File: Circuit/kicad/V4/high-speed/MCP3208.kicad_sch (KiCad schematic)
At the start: 15 parts, among them J16 Conn_01x02_Pin, J17 Conn_01x02_Pin, J18 Conn_01x02_Pin, J19 Conn_01x02_Pin, J20 Conn_01x02_Pin, J21 Conn_01x02_Pin, U24 MCP3208

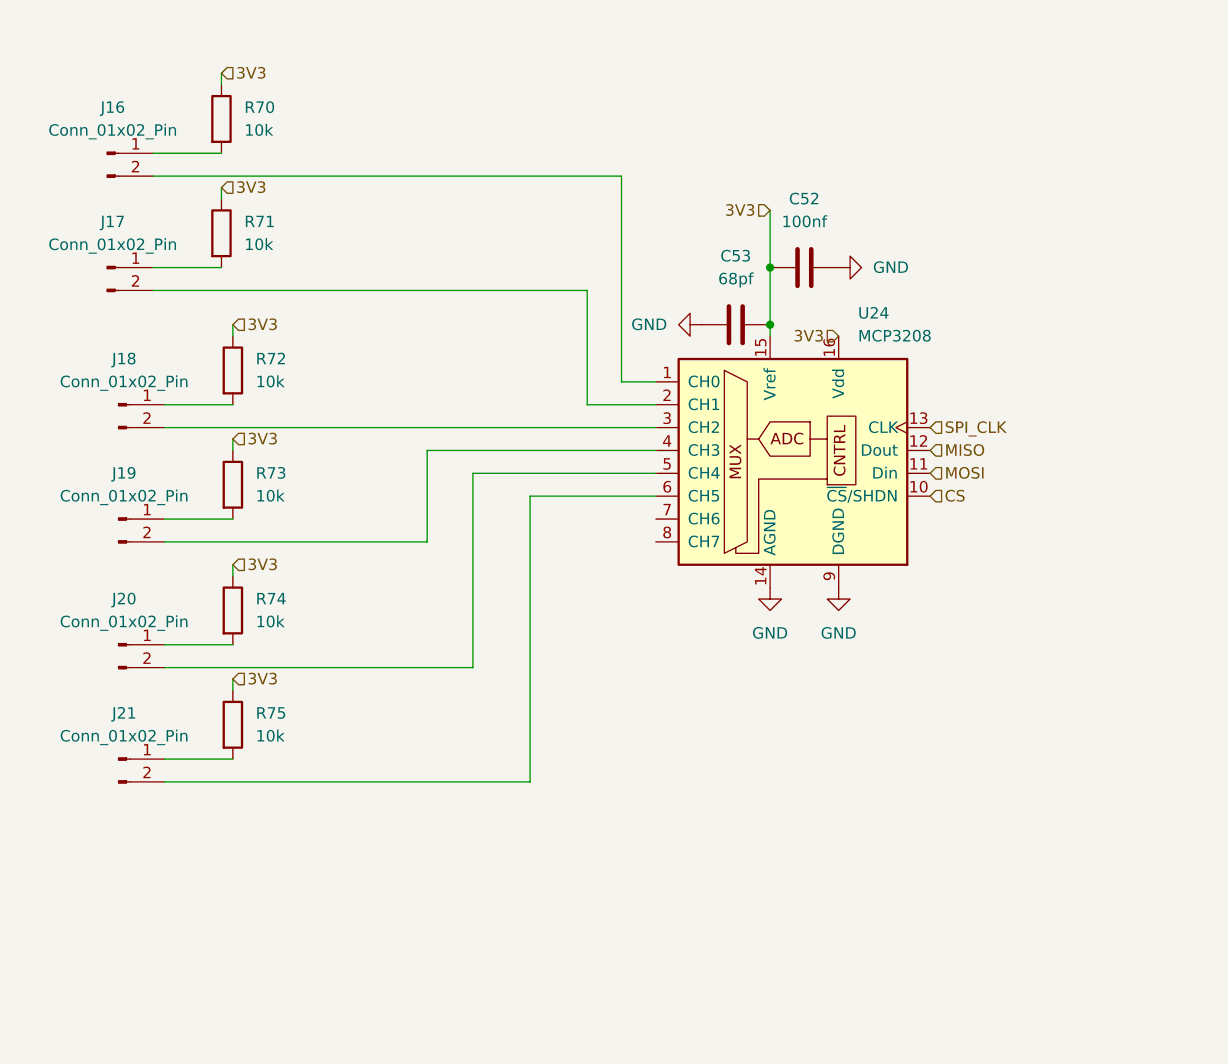
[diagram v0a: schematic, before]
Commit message: kicad: high speed V2.2 Circuit finish psu bom update
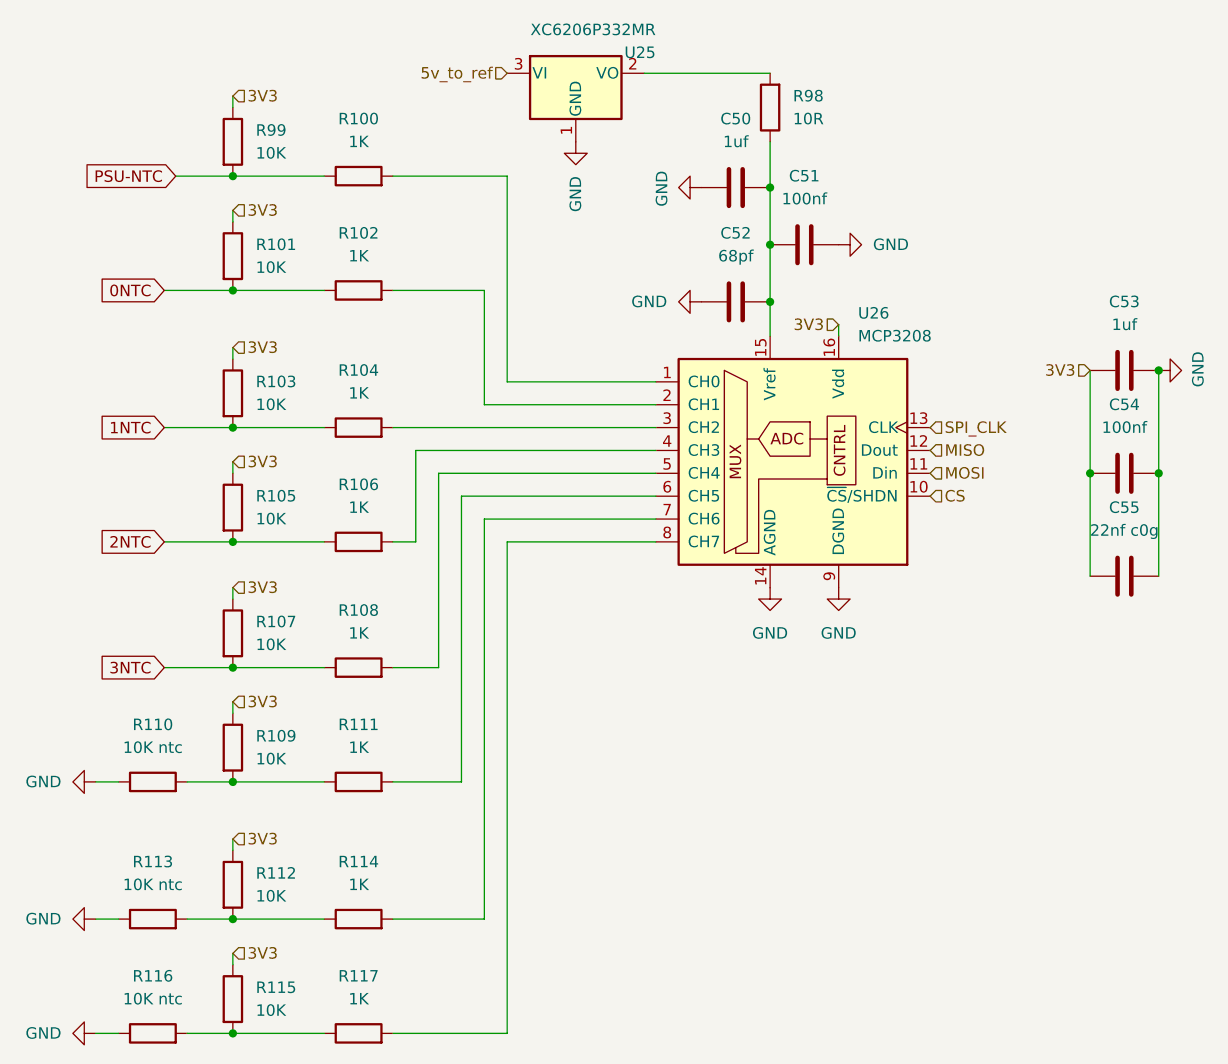
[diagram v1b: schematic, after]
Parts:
- removed J16, J17, J18, J19, J20, J21: Conn_01x02_Pin, Connector_PinHeader_2.54mm:PinHeader_2x01_P2.54mm_Vertical, symbol Connector:Conn_01x02_Pin
- added C50, C53: 1uf, Capacitor_SMD:C_0805_2012Metric, symbol Device:C
- added C54: 100nf, Capacitor_SMD:C_0805_2012Metric, symbol Device:C
- added C55: 22nf c0g, Capacitor_SMD:C_0805_2012Metric, symbol Device:C
- added R100, R102, R104, R106, R108, R111, R114, R117: 1K, Resistor_SMD:R_0805_2012Metric, symbol Device:R
- added R110, R113, R116: 10K ntc, Resistor_SMD:R_0805_2012Metric, symbol Device:R
- added R112, R115: 10K, Resistor_SMD:R_0805_2012Metric, symbol Device:R
- added R98: 10R, Resistor_SMD:R_0805_2012Metric, symbol Device:R
- added U25: XC6206P332MR, Package_TO_SOT_SMD:SOT-23-3, symbol Regulator_Linear:XC6206PxxxMR
- C51: renamed from C52; Cikkszám (none) -> 100.011.22; Link (none) -> https://www.hestore.hu/prod_10001122.html
- C52: renamed from C53; Cikkszám (none) -> 100.380.72; Link (none) -> https://www.hestore.hu/prod_10038072.html
- R101: renamed from R71; value 10k -> 10K; Cikkszám (none) -> 100.011.45; Link (none) -> https://www.hestore.hu/prod_10001145.html
- R103: renamed from R72; value 10k -> 10K; Cikkszám (none) -> 100.011.45; Link (none) -> https://www.hestore.hu/prod_10001145.html
- R105: renamed from R73; value 10k -> 10K; Cikkszám (none) -> 100.011.45; Link (none) -> https://www.hestore.hu/prod_10001145.html
- R107: renamed from R74; value 10k -> 10K; Cikkszám (none) -> 100.011.45; Link (none) -> https://www.hestore.hu/prod_10001145.html
- R109: renamed from R75; value 10k -> 10K; Cikkszám (none) -> 100.011.45; Link (none) -> https://www.hestore.hu/prod_10001145.html
- R99: renamed from R70; value 10k -> 10K; Cikkszám (none) -> 100.011.45; Link (none) -> https://www.hestore.hu/prod_10001145.html
- U26: renamed from U24; Cikkszám (none) -> 100.491.18; Link (none) -> https://www.hestore.hu/prod_10049118.html
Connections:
- net 3V3: now also C53.1, C54.1, C55.1, R112.1, R115.1; no longer C51.1, C52.2, U26.15 (Vref)
- net GND: now also C50.1, C53.2, C54.2, C55.2, R110.1, R113.1, R116.1, U25.1 (GND)
- net 0NTC: now reaches R101.2
- net 0NTC: now also R102.1
- net PSU-NTC: now reaches R99.2
- net PSU-NTC: now also R100.1
- net 3NTC: now reaches R107.2
- net 3NTC: now also R108.1
- net at U26.5 (CH4): now also R108.2
- net at R109.2: now also R110.2, R111.1
- net at U26.6 (CH5): now also R111.2
- net 1NTC: now reaches R103.2
- net 1NTC: now also R104.1
- net at U26.2 (CH1): now also R102.2
- net at U26.1 (CH0): now also R100.2
- net at U26.3 (CH2): now also R104.2
- net at U26.4 (CH3): now also R106.2
- net at U26.7 (CH6): now also R114.2
- net at U26.8 (CH7): now also R117.2
- net 2NTC: now reaches R105.2
- net 2NTC: now also R106.1
- new net: C50.2, C51.1, C52.2, R98.1, U26.15 (Vref)
- new net: R115.2, R116.2, R117.1
- new net: R98.2, U25.2 (VO)
- new net: R112.2, R113.2, R114.1
- new net 5v_to_ref: U25.3 (VI)
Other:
- moved on the sheet: C51, C52, R101, R103, R105, R107, R109, R99
